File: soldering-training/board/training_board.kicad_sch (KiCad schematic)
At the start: 23 parts, among them J1 MAIN_PWR, Q2 ARDUINOR3-NOIOREF-NOTEXT, SW1 PTS645, U2 DRV8876PWPRPWP0016J_NV

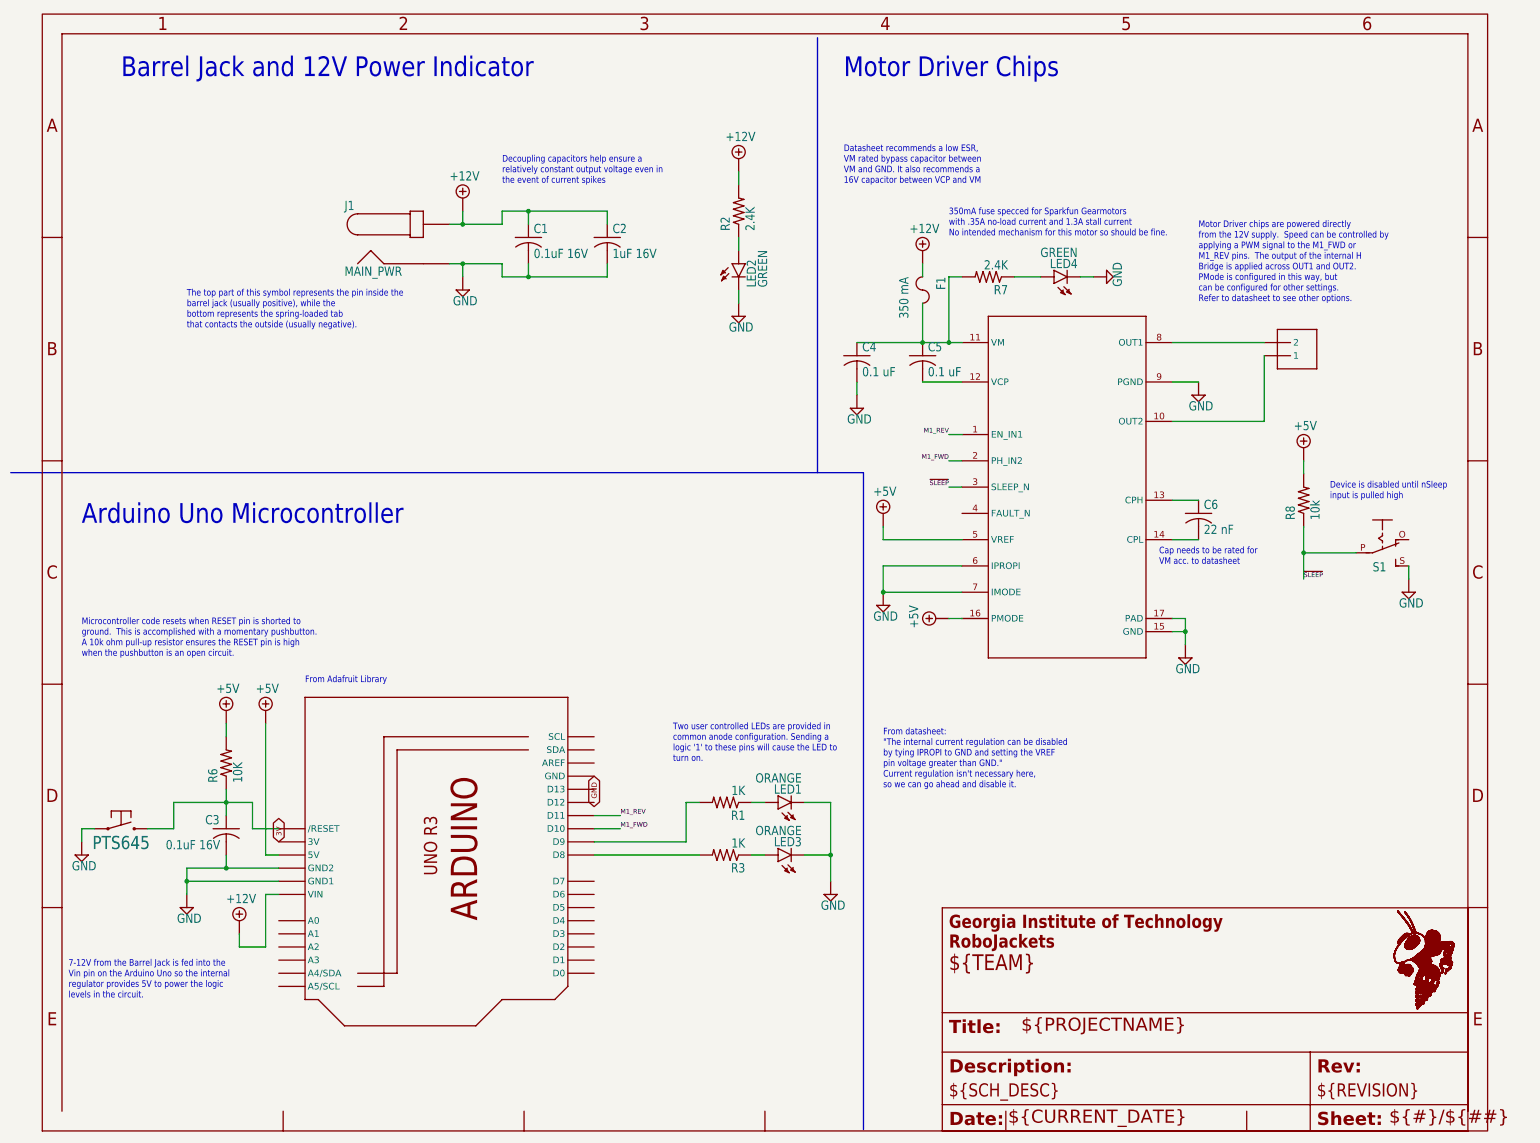
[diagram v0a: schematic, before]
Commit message: Add solution to week 4 lab and finish conversion of soldering training board from EAGLE to KiCAD
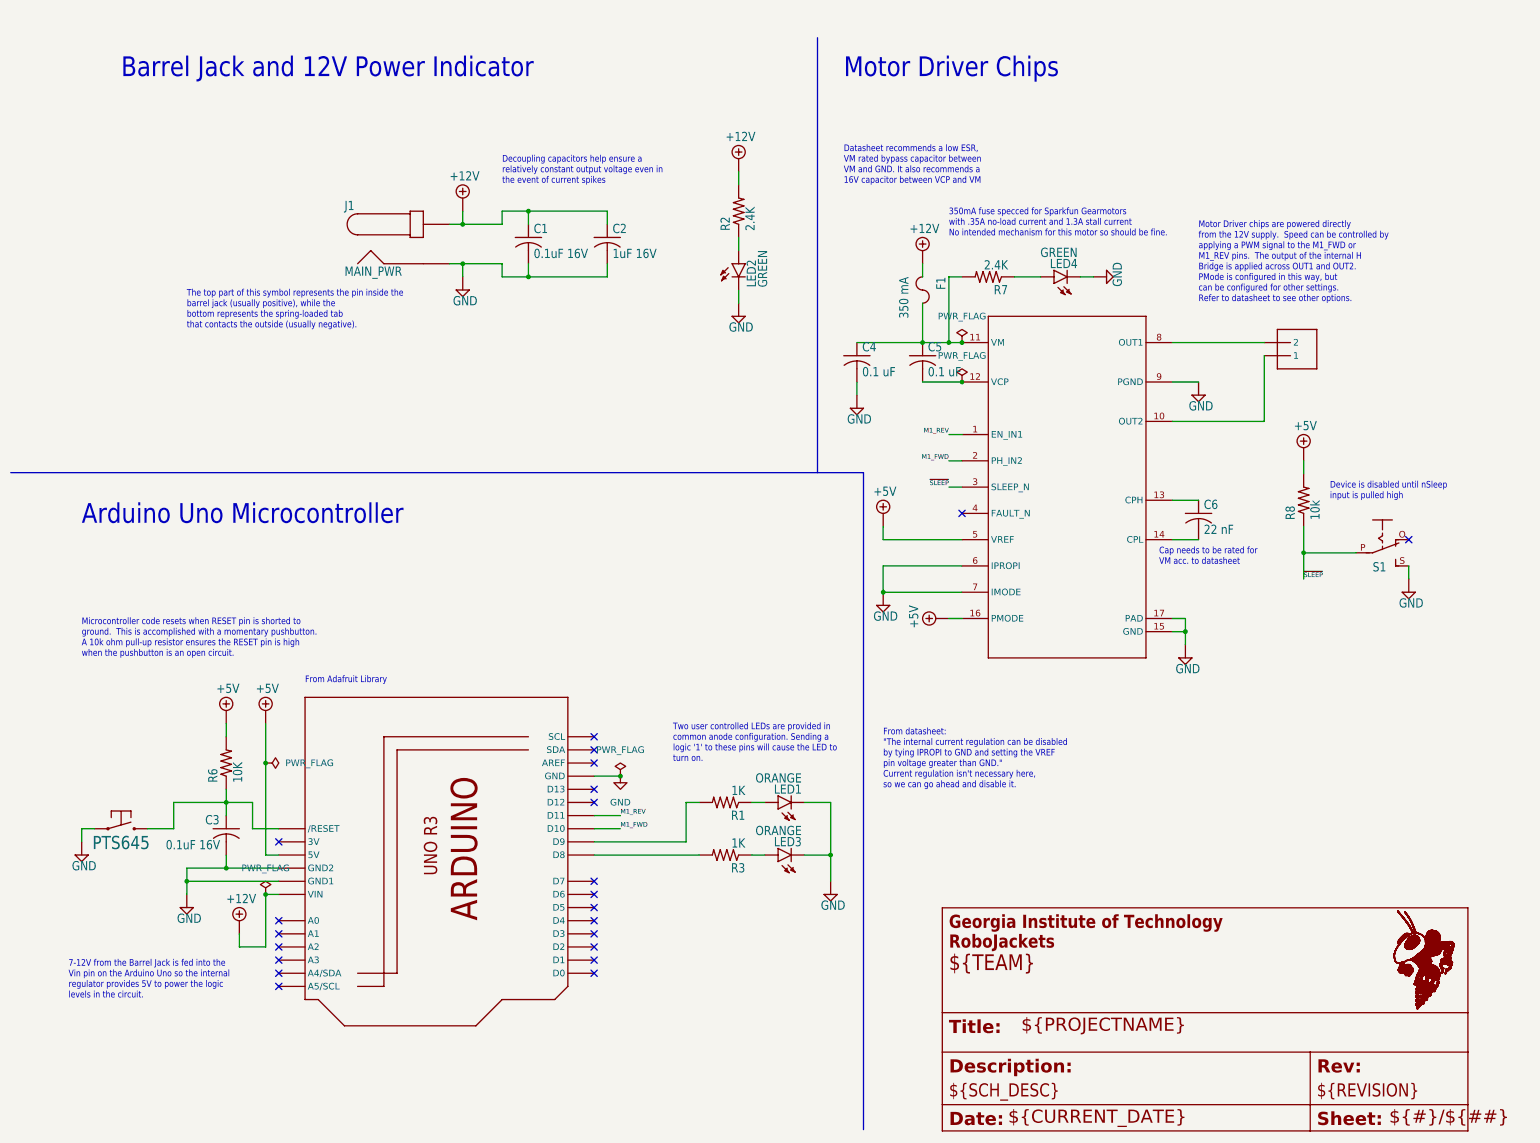
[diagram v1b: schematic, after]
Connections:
- net 3V: no longer names the net of Q2.3V
- no-connect marks 0 -> 22
